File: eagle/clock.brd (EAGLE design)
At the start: 74 x 33 mm, 17 parts, among them IC1 LM1117MPX-3.3

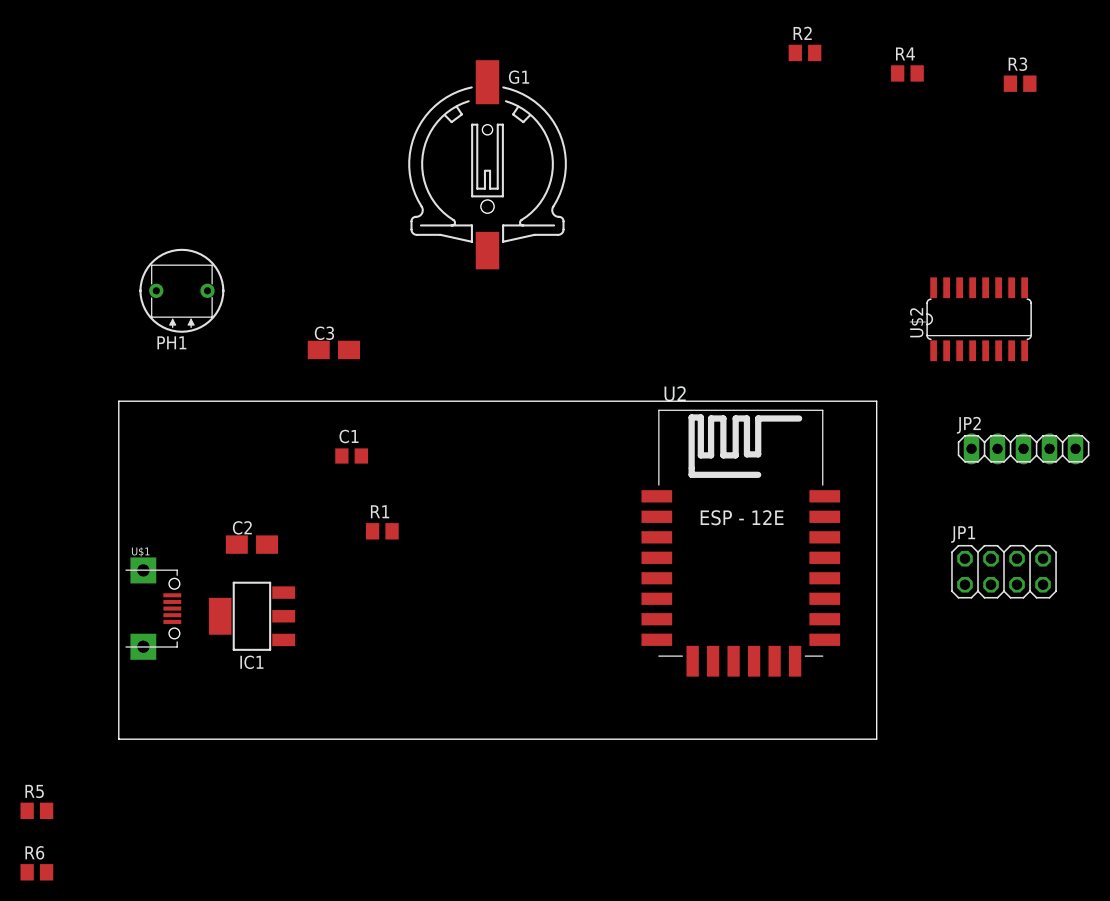
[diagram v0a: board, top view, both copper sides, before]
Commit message: First version of board design
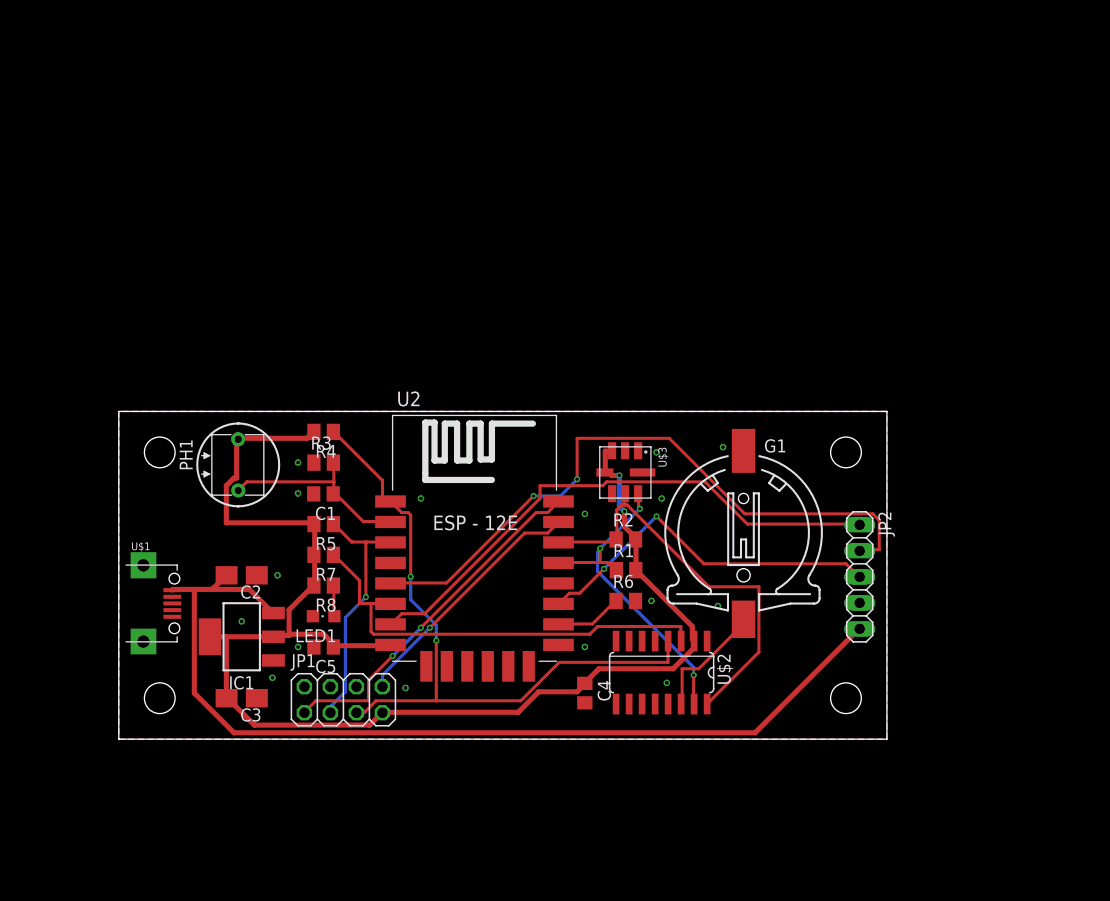
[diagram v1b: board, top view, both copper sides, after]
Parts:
- added C4, C5: 100u, rcl:C0805
- added LED1: G, led:CHIPLED_0805
- added R7: 4.7k, rcl:M0805
- added R8: 330, rcl:M0805
- added U$3: BMP085, bmp085:BMP085
- C1: value (none) -> 100u
- R1, R2, R4, R5, R6: value (none) -> 4.7k
- R3: value (none) -> 68k
- U2: value (none) -> ESP12E
- moved R3 77.4 mm to (20.0, 27.0)
- moved R4 66.9 mm to (20.0, 30.0), turned to 180 degrees
- moved JP1 65.7 mm to (21.9, 3.85)
- moved R6 63.3 mm to (49.5, 13.5)
- moved R2 50.6 mm to (49.5, 19.5)
- moved U$2 46.4 mm to (53.0, 6.50), turned to 180 degrees
- moved G1 43.8 mm to (61.0, 14.0)
- moved R5 39.6 mm to (20.0, 21.0), turned to 180 degrees
- moved C3 35.2 mm to (12.0, 4.00), turned to 180 degrees
- moved U2 26.0 mm to (34.8, 17.4)
- moved R1 24.1 mm to (49.5, 16.5)
- moved JP2 20.3 mm to (72.3, 15.8), turned to 270 degrees
- moved PH1 17.9 mm to (11.7, 26.8), turned to 270 degrees
- moved C1 4.61 mm to (20.0, 23.9), turned to 180 degrees
- moved C2 3.16 mm to (12.0, 16.0), turned to 180 degrees
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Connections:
- net N$1 renamed VBAT
- net N$2 renamed GPIO15
- net +3V3: now also C4.1, C5.1, JP1.7, R7.2, R8.2, U$2.2, U$3.3, U$3.4
- net DSP_CLK: now also U2.GPIO14
- net DSP_CS: now also U2.GPIO2
- net DSP_DIN: now also U2.GPIO13
- net GND: now also C4.2, C5.2, LED1.C, U$3.1
- net N$3: now also LED1.A, R8.1; no longer U$2.2
- net SCL: now also U$3.6, U2.GPIO5
- net SDA: now also U$3.7, U2.GPIO4
- net TIMER_INT: now also R7.1, U2.GPIO12
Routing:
- net +3V3: track 0.00 -> 135.9 mm, vias 0 -> 2
- net +5V: track 0.00 -> 93.7 mm
- net RESET: track 0.00 -> 65.8 mm, vias 0 -> 2
- net DSP_CLK: track 0.00 -> 64.1 mm, vias 0 -> 2
- net DSP_DIN: track 0.00 -> 54.0 mm
- net TIMER_INT: track 0.00 -> 43.7 mm
- net SCL: track 0.00 -> 40.7 mm
- net DSP_CS: track 0.00 -> 35.4 mm, vias 0 -> 2
- net TX: track 0.00 -> 34.6 mm, vias 0 -> 2
- net SDA: track 0.00 -> 33.6 mm, vias 0 -> 3
- net RX: track 0.00 -> 24.5 mm, vias 0 -> 1
- net CH_PD: track 0.00 -> 24.4 mm, vias 0 -> 1
- net LIGHT_SENSOR: track 0.00 -> 19.6 mm
- net VBAT: track 0.00 -> 11.8 mm
- net GPIO15: track 0.00 -> 6.56 mm
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- added copper zone on layer 1, net GND
- added copper zone on layer 16, net GND
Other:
- board size 74 x 33 mm -> 75 x 32 mm
